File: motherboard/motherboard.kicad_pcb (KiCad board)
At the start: 2 copper layers, 85 x 56.5 mm, 29 parts, among them J1 Conn_01x02_Male, J2 Temp_connector, J3 24V_connector, P1 Raspberry_Pi_+_Conn, Q1 Q_NMOS_GSD, Q2 Q_NMOS_GSD, U1 74AUC2G04, U2 quad_and, U3 TLC272

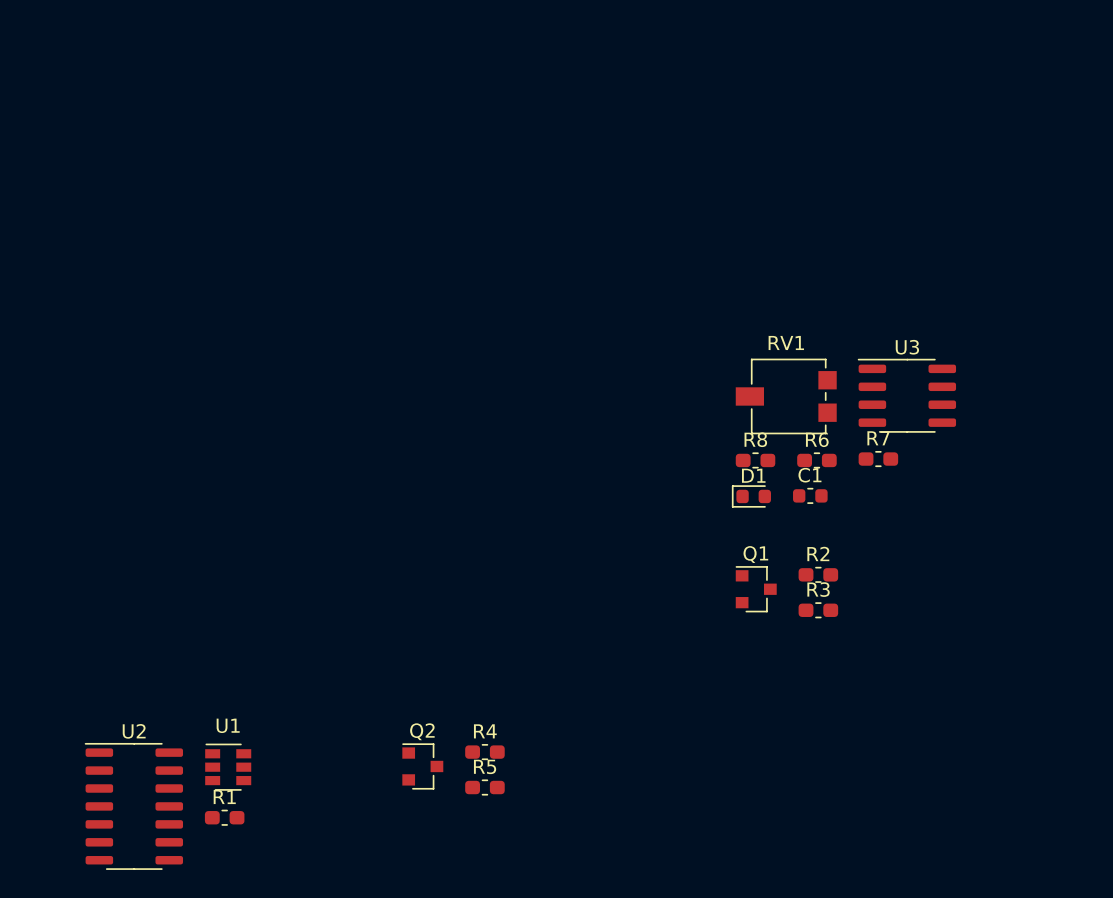
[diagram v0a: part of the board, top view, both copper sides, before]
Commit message: WIP: Motherboard v1.1
  Cosmetic changes
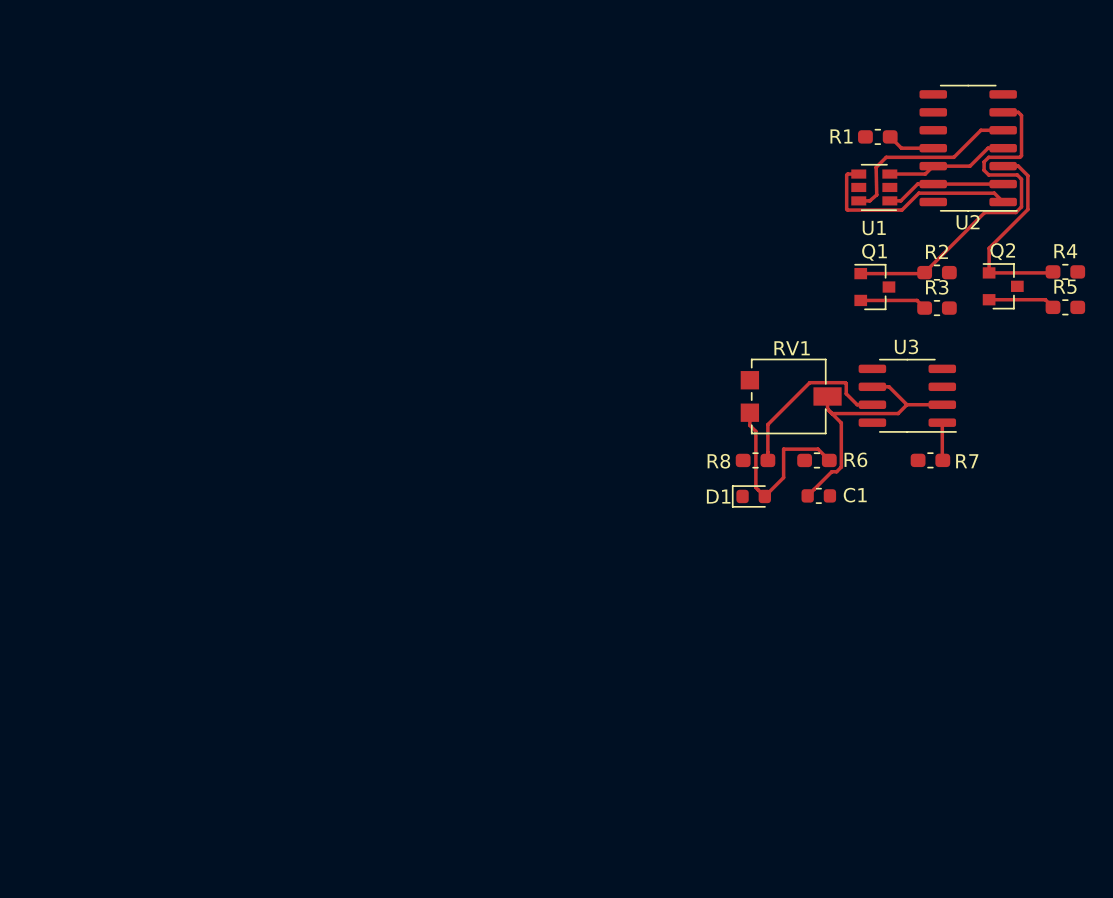
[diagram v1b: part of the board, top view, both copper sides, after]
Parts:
- moved U2 75.2 mm to (213.3, 55.6), turned to 180 degrees
- moved R1 66.8 mm to (206.9, 54.8)
- moved U1 61.5 mm to (206.6, 58.4), turned to 180 degrees
- moved Q2 53.3 mm to (215.8, 65.4)
- moved R4 53.3 mm to (220.2, 64.4)
- moved R5 53.3 mm to (220.2, 66.9)
- moved R2 23.0 mm to (211.1, 64.4)
- moved Q1 23.0 mm to (206.7, 65.4)
- moved R3 23.0 mm to (211.1, 66.9)
- moved R7 3.69 mm to (210.6, 77.7), turned to 180 degrees
- moved C1 0.60 mm to (202.7, 80.2)
- turned R8 to 180 degrees
- turned RV1 to 180 degrees
- turned U3 to 180 degrees
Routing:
- net Net-(R8-Pad1): track 41.9 -> 93.7 mm
- net Net-(C1-Pad1): track 18.8 -> 57.4 mm
- net /SSR_interface/SSR_driver_2/indicator: track 39.6 -> 4.75 mm
- net Net-(R7-Pad1): track 29.6 -> 2.68 mm
- net /SSR_interface/SSR_driver_1/sig_in: track 13.9 -> 39.7 mm
- net Net-(D1-Pad2): track 7.66 -> 32.7 mm
- net Net-(U1-Pad4): track 7.72 -> 22.9 mm
- net /SSR_interface/SSR_driver_2/sig_in: track 16.5 -> 31.1 mm
- net Net-(U1-Pad6): track 10.1 -> 23.6 mm
- net /SSR_interface/SSR2_GPIO: track 46.7 -> 55.5 mm
- net /SSR_interface/SSR1_GPIO: track 35.2 -> 43.7 mm
- net /SSR_interface/SSR_driver_1/indicator: track 30.5 -> 35.2 mm
- net Net-(R1-Pad2): track 36.3 -> 39.7 mm
